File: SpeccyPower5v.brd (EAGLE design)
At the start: 112.1 x 36.8 mm, 62 parts, among them T1 TRANS_ER29

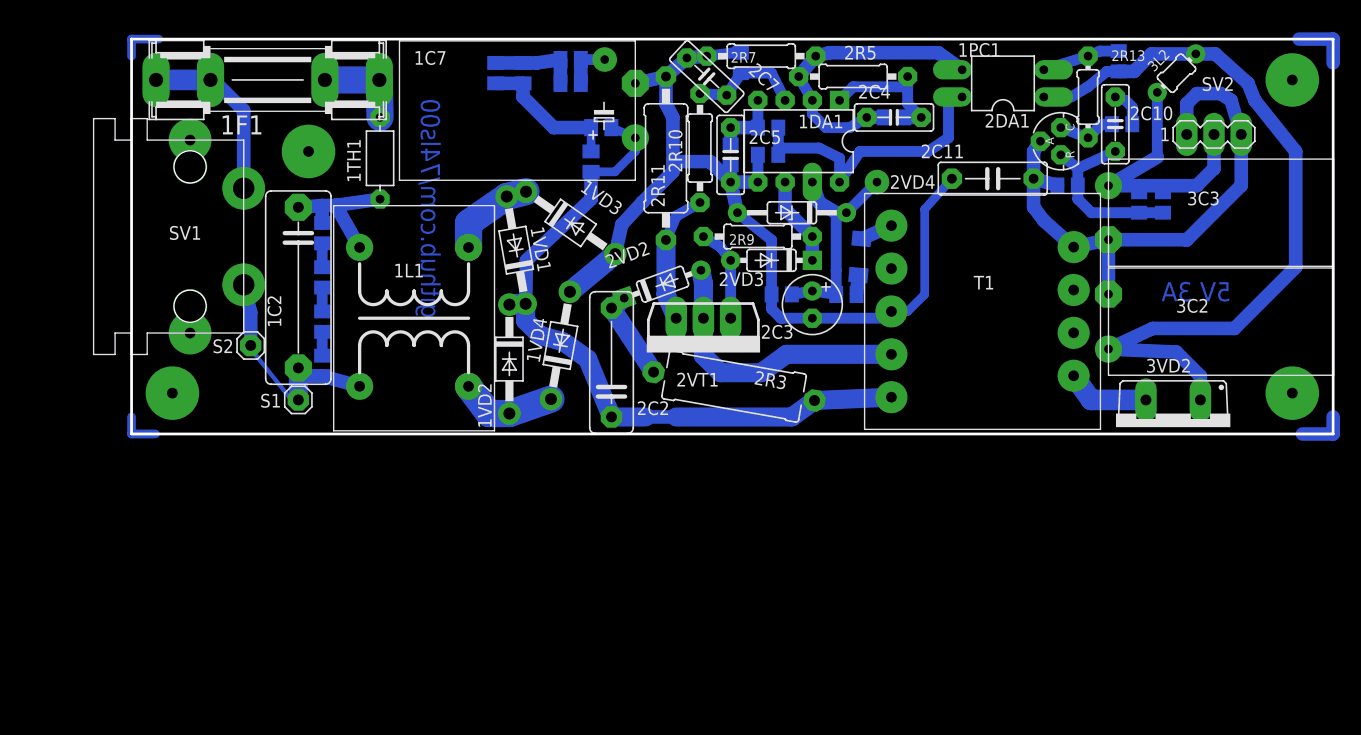
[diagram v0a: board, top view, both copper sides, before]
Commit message: ..
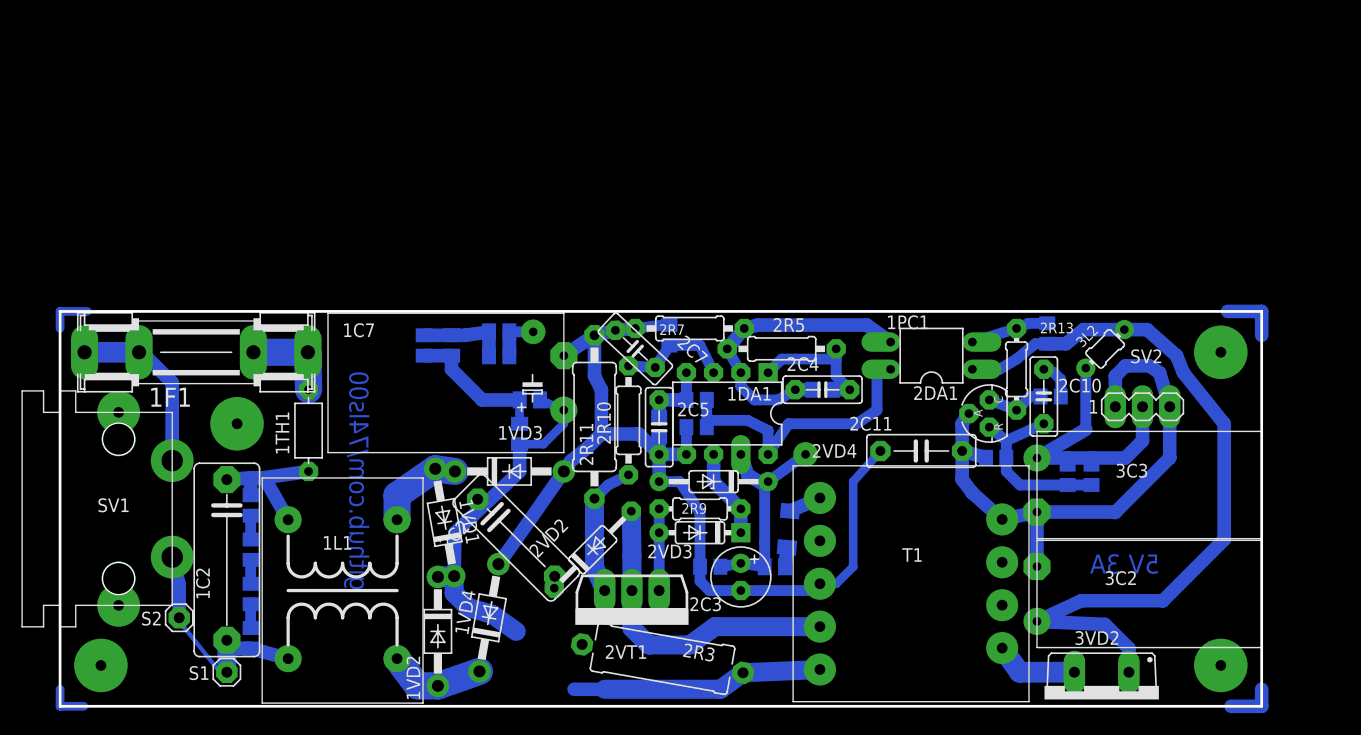
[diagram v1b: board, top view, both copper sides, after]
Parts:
- 2R9: device rcl:0207/10 -> rcl:0204/7
- 2VD2: device SpeccyPower5v:DO35-7 -> SpeccyPower5v:DO35-10
- moved 3L2 26.6 mm to (104.1, 43.8)
- moved 1C7 26.3 mm to (53.7, 40.6)
- moved 1DA1 26.3 mm to (68.9, 37.8)
- moved 1TH1 26.3 mm to (29.8, 36.2)
- moved 1VD2 26.3 mm to (41.9, 17.5)
- moved 1VD4 26.3 mm to (46.7, 18.7)
- moved 2C10 26.3 mm to (98.4, 39.4)
- moved 2C4 26.3 mm to (77.8, 40.0)
- moved 2C4A 26.3 mm to (77.8, 40.0)
- moved 2C5 26.3 mm to (62.5, 36.5)
- moved 2C5A 26.3 mm to (62.5, 36.5)
- moved 2C7 26.3 mm to (60.3, 43.8)
- moved 2C7A 26.3 mm to (63.5, 45.1)
- moved 2DA1 26.3 mm to (93.3, 37.8)
- moved 2R10 26.3 mm to (59.7, 37.1)
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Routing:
- net +IN: track 66.0 -> 57.0 mm
- net N$30: track 8.65 -> 1.11 mm
- net N$17: track 26.7 -> 29.6 mm
- net -IN: track 88.4 -> 89.9 mm
- net N$11: track 8.84 -> 7.62 mm
- net +16IN: track 25.8 -> 25.3 mm
